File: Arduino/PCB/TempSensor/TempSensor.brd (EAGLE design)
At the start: 32.7 x 32.4 mm, 24 parts, among them IC1 DS1820, J1 FTDI_DEVICE, J2 FTDI_DEVICE, U1 ATMEGA328-AU, X1 16Mhz

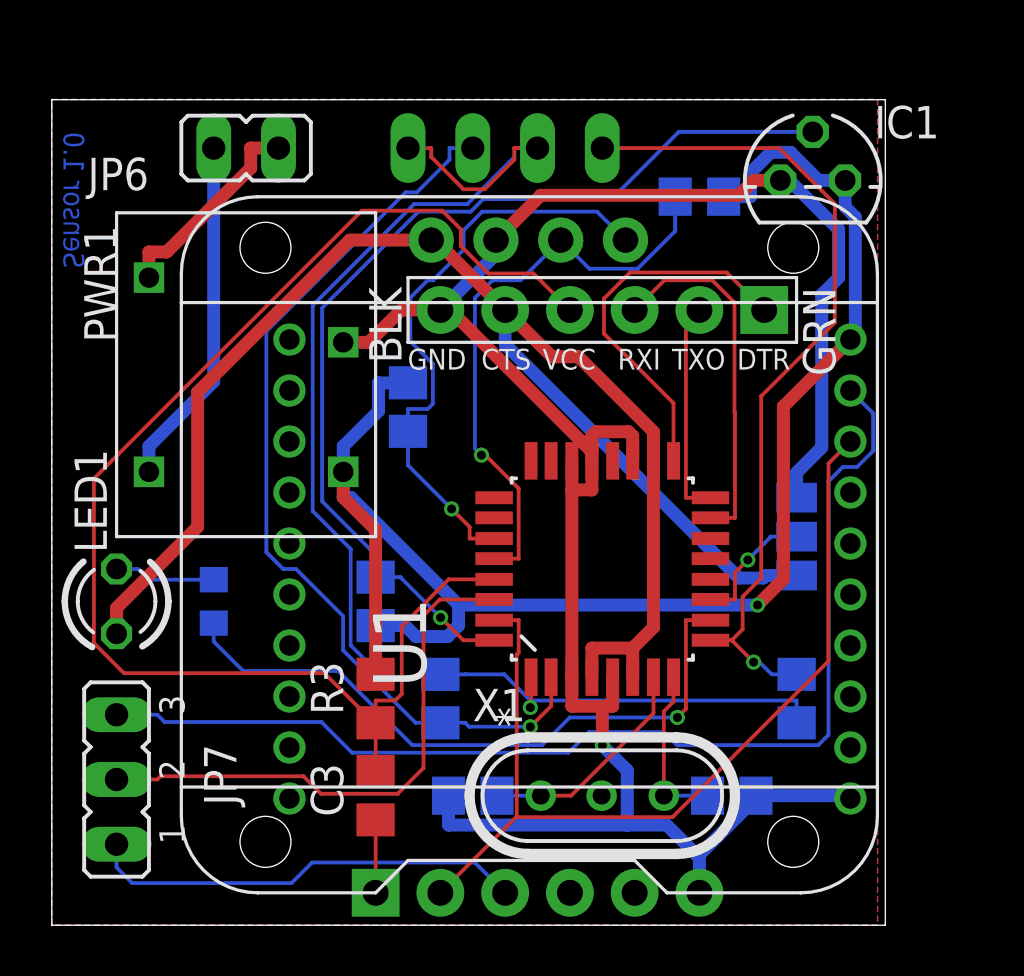
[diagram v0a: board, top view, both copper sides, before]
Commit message: base board
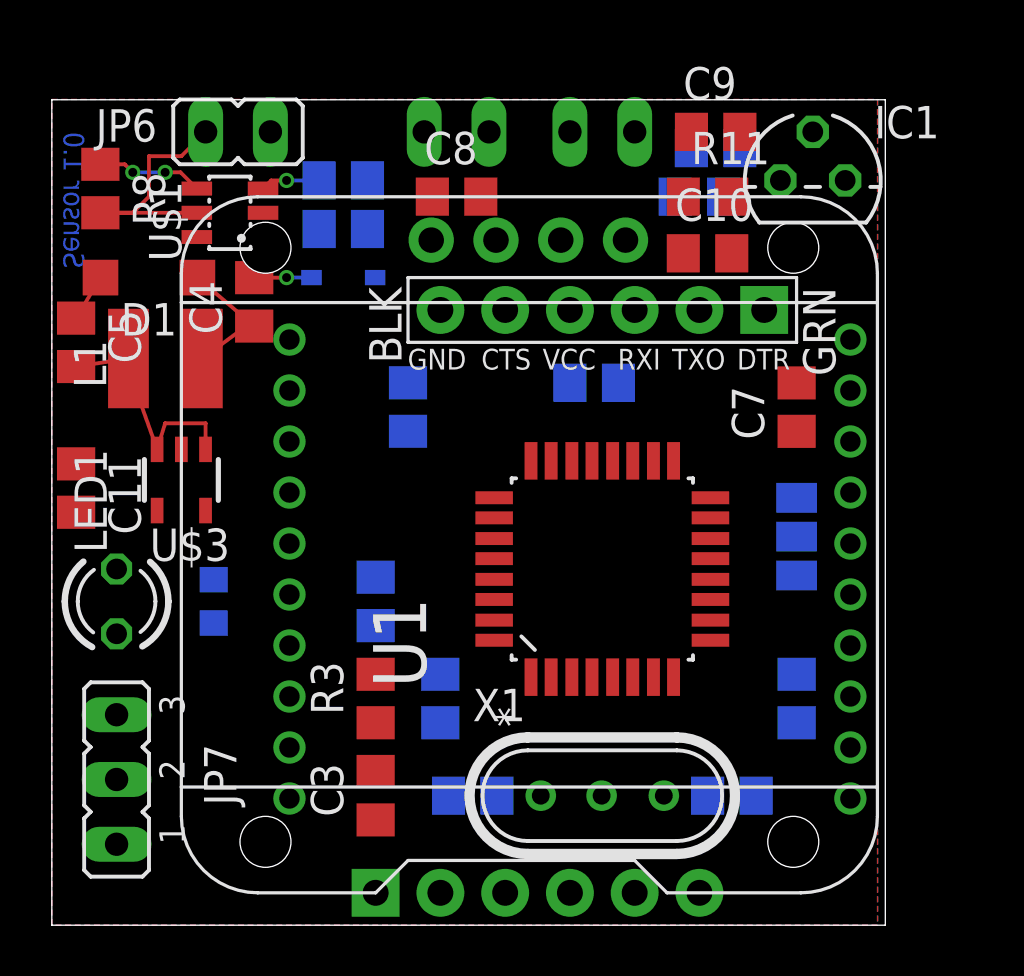
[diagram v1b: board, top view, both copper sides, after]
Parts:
- removed PWR1: IE0503D, xp_power:XP_DIP
- added C10, C4, C5, C6, C7, C8, C9: 100n, rcl:C0805
- added C11: 10n, rcl:C0805
- added D1: RB161M-20TR, Components:SOD123
- added D2: BAT54HT1G, Components:SOD323_ST
- added L1: VLCF4020, Components:VLCF4020
- added R10, R11, R13, R9: 4k7, rcl:R0805
- added R8: 10k, rcl:R0805
- added U$1: LM2736X, Components:SOT23-6L
- added U$3: XC6210, Components:SOT23-5
- U$2: value OLED_0.96_I2C -> OLED_0.96_I2CSWITCHPOWER
- moved JP5 1.42 mm to (58.4, 51.4)
- moved JP4 0.90 mm to (52.7, 51.4)
- moved JP6 0.71 mm to (44.1, 51.4)
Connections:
- removed net VCC: J2.P$5, LED1.A, SJ2.1, U$2.VCC, U1.18, U1.4, U1.6
- new net N$19: C4.2, D2.C, U$1.1
- new net N$25: R8.1, U$1.4
- new net N$26: C9.2, IC1.3, R11.1
- new net N$27: C10.2, IC1.2, R13.1
- new net N$29: C11.2, U$3.4
- new net VIN: JP6.2, R8.2, U$1.5
- new net VO: C5.2, D2.A, L1.P$2, R9.2, U$3.1, U$3.3
- net +3V3: now also C6.2, C7.2, C8.2, J2.P$5, LED1.A, R11.2, SJ2.1, U$2.GND, U$3.5, U1.18, U1.4, U1.6; no longer IC1.3, PWR1.+VOUT
- net GND: now also C10.1, C11.1, C5.1, C6.1, C7.1, C8.1, C9.1, D1.A, JP6.1, R10.1, U$1.2, U$2.VCC, U$3.2; no longer PWR1.-VOUT, U$2.GND
- net N$11: now also C4.1, D1.C, L1.P$1, U$1.6; no longer JP6.2, PWR1.+VIN
- net N$14: now also R10.2, R9.1, U$1.3; no longer JP6.1, PWR1.-VIN
- net N$6: now also R13.2; no longer IC1.2
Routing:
- net GND: track 85.6 -> 1.86 mm, vias 1 -> 0
- net VCC: track 63.6 -> 0.00 mm
- net +3V3: track 62.0 -> 0.00 mm, vias 1 -> 0
- net N$20: track 54.6 -> 0.00 mm
- net N$10: track 53.3 -> 0.00 mm, vias 1 -> 0
- net N$18: track 44.2 -> 0.00 mm
- net N$6: track 39.2 -> 0.00 mm, vias 1 -> 0
- net N$5: track 36.7 -> 0.00 mm
- net N$12: track 36.3 -> 0.00 mm, vias 1 -> 0
- net N$13: track 32.8 -> 0.00 mm, vias 1 -> 0
- net N$16: track 26.0 -> 0.00 mm, vias 1 -> 0
- net N$8: track 23.4 -> 0.00 mm, vias 1 -> 0
- net N$9: track 23.2 -> 0.00 mm, vias 1 -> 0
- net N$4: track 21.8 -> 0.00 mm
- net N$3: track 17.2 -> 0.00 mm
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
